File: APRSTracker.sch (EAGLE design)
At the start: 27 parts, among them IC1 TP4056, X1 POWERSUPPLY_DC21MMX

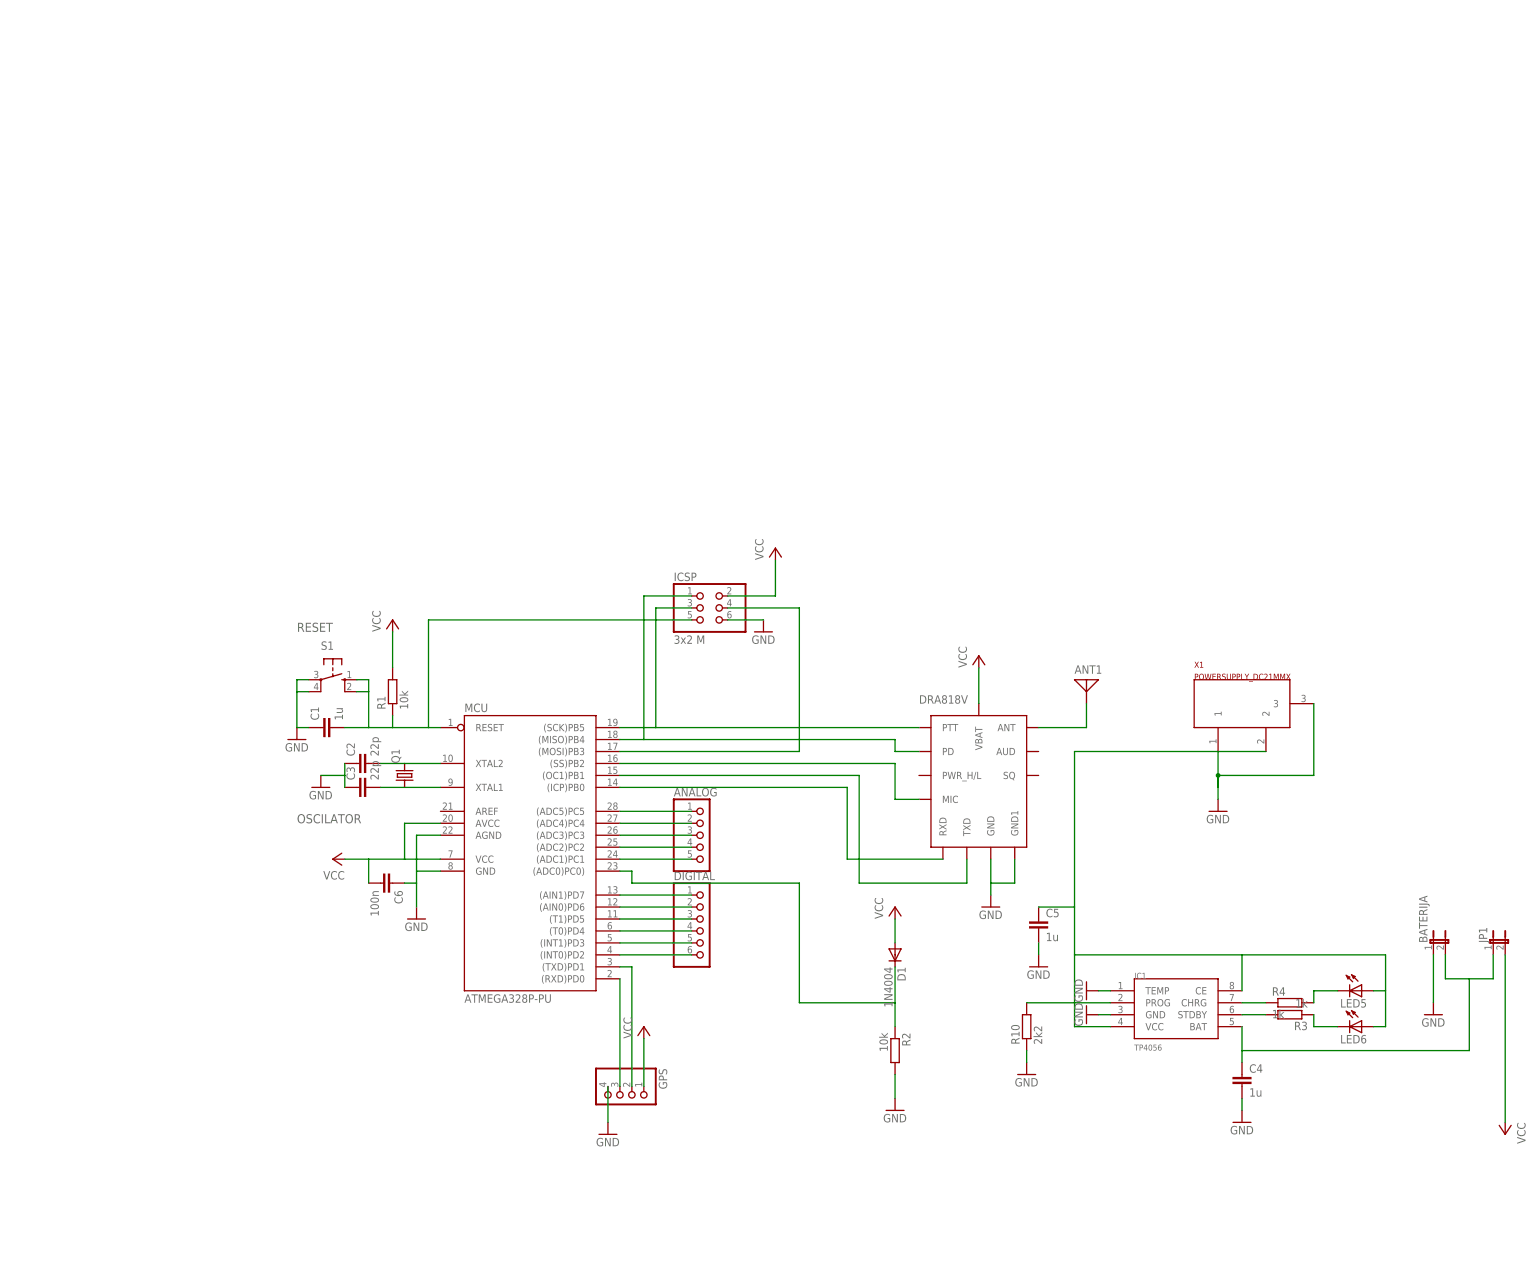
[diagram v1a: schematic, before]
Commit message: shema v2
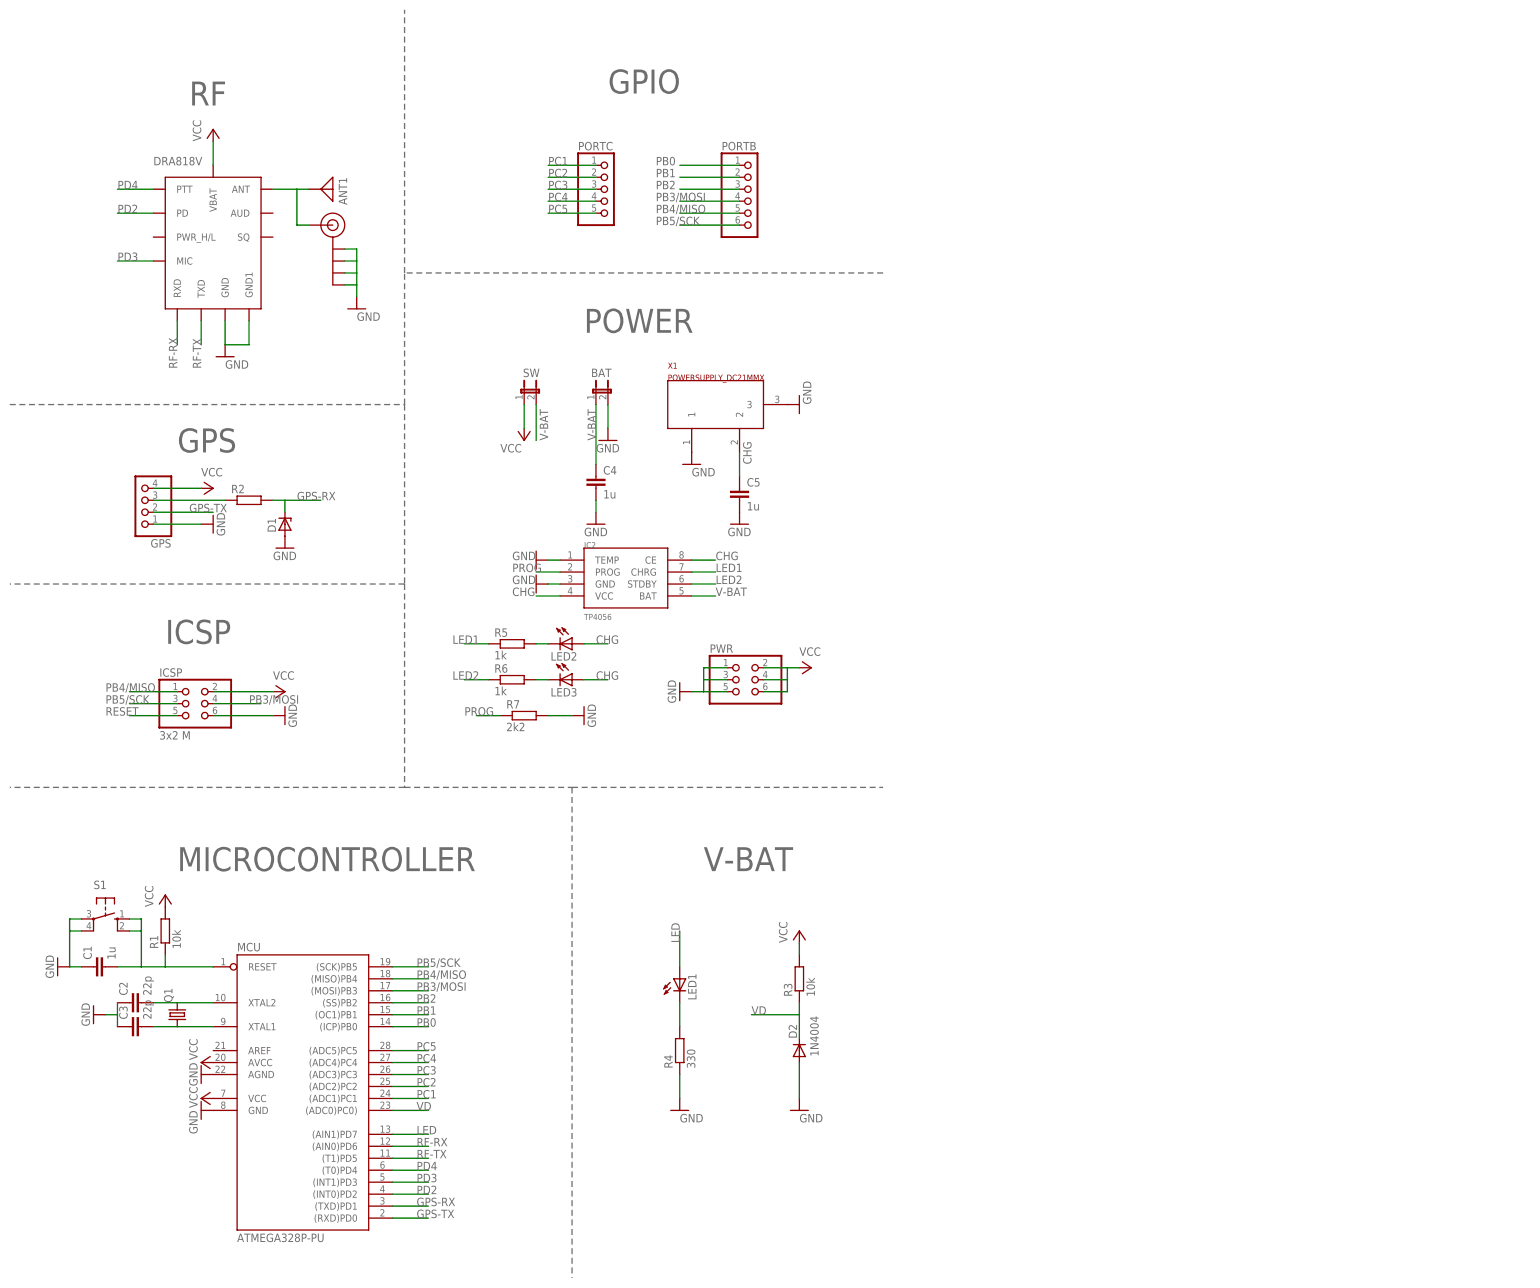
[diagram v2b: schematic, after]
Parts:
- removed ANALOG: (no value), pinhead:PINHD-1X5
- removed BATERIJA, JP1: (no value), jumper:JP1E
- removed C6: 100n, rcl:C-EU050-024X044
- removed DIGITAL: (no value), pinhead:PINHD-1X6
- removed IC1: TP4056, TP4056:TP4056
- removed LED5, LED6: (no value), led:LED3MM
- removed R10: 2k2, rcl:R-EU_0207/10
- added ANT: SMA_EDGE, SparkFun:SMA_EDGE
- added BAT, SW: (no value), jumper:JP1E
- added D2: 1N4004, diode1:1N4004
- added IC2: TP4056, TP4056:TP4056
- added LED1, LED2, LED3: (no value), led:LED3MM
- added PORTB: (no value), pinhead:PINHD-1X6
- added PORTC: (no value), pinhead:PINHD-1X5
- added PWR: (no value), pinhead:PINHD-2X3
- added R5, R6: 1k, rcl:R-EU_0207/10
- added R7: 2k2, rcl:R-EU_0207/10
- D1: value 1N4004 -> (none); device diode:1N4004 -> diode:ZENER-DIODEDO35Z10
- R2: value 10k -> (none)
- R3: value 1k -> 10k
- R4: value 1k -> 330
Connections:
- net N$4 renamed RESET
- removed net N$10: ANT1.1, DRA818V.ANT
- removed net N$11: DRA818V.TXD, MCU.(OC1)PB1
- removed net N$12: DRA818V.RXD, MCU.(ICP)PB0
- removed net N$13: ANALOG.1, MCU.(ADC5)PC5
- removed net N$14: D1.C, MCU.(ADC0)PC0), R2.1
- removed net N$15: ANALOG.2, MCU.(ADC4)PC4
- removed net N$16: ANALOG.3, MCU.(ADC3)PC3
- removed net N$17: ANALOG.4, MCU.(ADC2)PC2
- removed net N$18: IC1.CHRG, R4.1
- removed net N$19: ANALOG.5, MCU.(ADC1)PC1
- removed net N$20: DIGITAL.1, MCU.(AIN1)PD7
- removed net N$21: DIGITAL.2, MCU.(AIN0)PD6
- removed net N$22: DIGITAL.3, MCU.(T1)PD5
- removed net N$23: IC1.STDBY, R3.2
- removed net N$24: LED5.C, R4.2
- removed net N$25: LED6.C, R3.1
- removed net N$26: IC1.PROG, R10.2
- removed net N$27: C5.1, IC1.CE, IC1.VCC, LED5.A, LED6.A, X1.2
- removed net N$28: DIGITAL.4, MCU.(T0)PD4
- removed net N$29: DIGITAL.5, MCU.(INT1)PD3
- removed net N$30: DIGITAL.6, MCU.(INT0)PD2
- removed net N$31: BATERIJA.2, C4.1, IC1.BAT, JP1.1
- removed net N$8: GPS.3, MCU.(RXD)PD0
- removed net N$9: DRA818V.MIC, MCU.(SS)PB2
- new net CHG: C5.1, IC2.CE, IC2.VCC, LED2.A, LED3.A, X1.2
- new net GPS-RX: D1.C, MCU.(TXD)PD1, R2.2
- new net GPS-TX: GPS.2, MCU.(RXD)PD0
- new net LED: LED1.A, MCU.(AIN1)PD7
- new net LED1: IC2.CHRG, R5.1
- new net LED2: IC2.STDBY, R6.1
- new net N$4: LED2.C, R5.2
- new net PB0: MCU.(ICP)PB0, PORTB.1
- new net PB1: MCU.(OC1)PB1, PORTB.2
- new net PB2: MCU.(SS)PB2, PORTB.3
- new net PB3/MOSI: ICSP.4, MCU.(MOSI)PB3, PORTB.4
- new net PB4/MISO: ICSP.1, MCU.(MISO)PB4, PORTB.5
- new net PB5/SCK: ICSP.3, MCU.(SCK)PB5, PORTB.6
- new net PC1: MCU.(ADC1)PC1, PORTC.1
- new net PC2: MCU.(ADC2)PC2, PORTC.2
- new net PC3: MCU.(ADC3)PC3, PORTC.3
- new net PC4: MCU.(ADC4)PC4, PORTC.4
- new net PC5: MCU.(ADC5)PC5, PORTC.5
- new net PD2: DRA818V.PD, MCU.(INT0)PD2
- new net PD3: DRA818V.MIC, MCU.(INT1)PD3
- new net PD4: DRA818V.PTT, MCU.(T0)PD4
- new net PROG: IC2.PROG, R7.1
- new net RF-RX: DRA818V.RXD, MCU.(AIN0)PD6
- new net RF-TX: DRA818V.TXD, MCU.(T1)PD5
- new net V-BAT: BAT.1, C4.1, IC2.BAT, SW.2
- new net VD: D2.C, MCU.(ADC0)PC0), R3.1
- net GND: now also ANT.GND@0, ANT.GND@1, ANT.GND@2, ANT.GND@3, BAT.2, D1.A, D2.A, GPS.1, IC2.GND, IC2.TEMP, PWR.1, PWR.3, PWR.5, R4.1, R7.2; no longer BATERIJA.1, C6.1, GPS.4, IC1.GND, IC1.TEMP, R10.1, R2.2
- net N$1: now also ANT.SIGNAL, ANT1.1, DRA818V.ANT; no longer ICSP.4, MCU.(MOSI)PB3
- net N$2: now also GPS.3, R2.1; no longer DRA818V.PD, ICSP.1, MCU.(MISO)PB4
- net N$3: now also LED1.C, R4.2; no longer DRA818V.PTT, ICSP.3, MCU.(SCK)PB5
- net N$7: now also LED3.C, R6.2; no longer GPS.2, MCU.(TXD)PD1
- net VCC: now also GPS.4, PWR.2, PWR.4, PWR.6, R3.2, SW.1; no longer C6.2, D1.A, GPS.1, JP1.2
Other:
- note added: "GPIO"
- note added: "GPS"
- note added: "ICSP"
- note added: "MICROCONTROLLER"
- note added: "POWER"
- note added: "RF"
- note added: "V-BAT"
- note removed: "OSCILATOR"
- note removed: "RESET"
- moved on the sheet: ANT1, C1, C2, C3, C4, C5, DRA818V, GPS, ICSP, MCU, Q1, R1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
